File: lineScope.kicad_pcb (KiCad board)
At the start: 2 copper layers, 100 x 60.6 mm, 95 parts, among them J1 Conn_01x02, J2 Conn_01x02, J3 Conn_01x03, J4 Conn_01x03, J5 Conn_01x03, J6 Conn_01x02, J7 Conn_Coaxial, J8 Conn_Coaxial, J9 Conn_01x04, K1 HE721A0500, K2 HE721A0500, Q1 BC847, Q2 BC847, U1 ADuM3190, U2 ADuM3190, U3 L78L09_SOT89, U4 LM4040DBZ-2.0, U5 L78L09_SOT89, U6 LM358

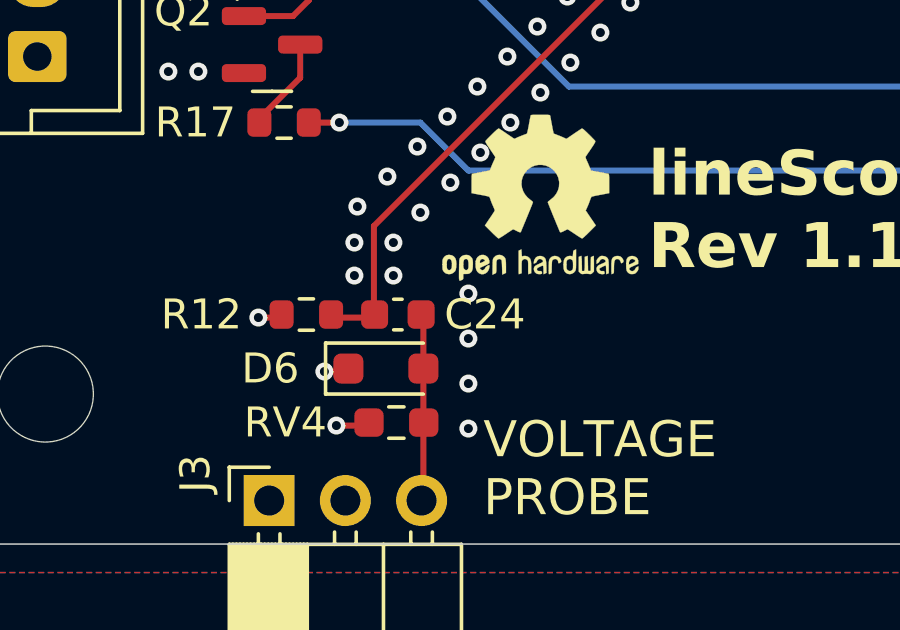
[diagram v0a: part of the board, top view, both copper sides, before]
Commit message: Fix C24
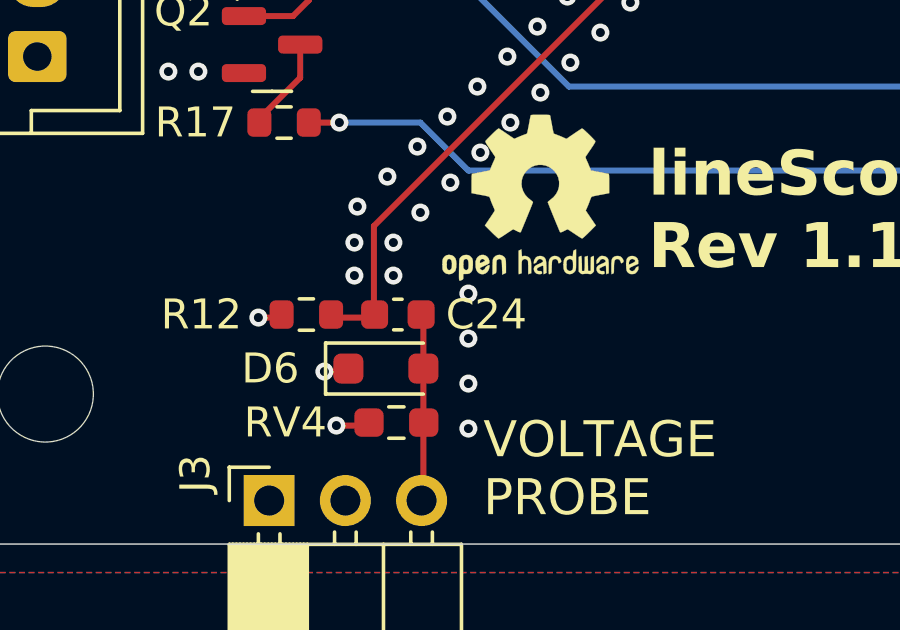
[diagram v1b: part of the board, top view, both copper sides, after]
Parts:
- J1, J2, J6: value Conn_01x02 -> B4B-XH-A(LF)(SN)
- turned C24 to 180 degrees
